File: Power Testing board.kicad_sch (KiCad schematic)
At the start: 5 parts, among them U1 INA260, U2 INA260, U3 INA260, U4 INA260

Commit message: GPT progress
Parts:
- removed A1: Arduino_Nano_Every, Module:Arduino_Nano, symbol MCU_Module:Arduino_Nano_Every
- removed U1, U2, U3, U4: INA260, Package_SO:TSSOP-16_4.4x5mm_P0.65mm, symbol Sensor:INA260
- added A1: Arduino Nano USB-powered socket, Module:Arduino_Nano, symbol Power_Testing_Board:Arduino_Nano_USB_Powered
- added C1, C3, C5, C7: 1uF input close to eFuse, Capacitor_SMD:C_0805_2012Metric, symbol Power_Testing_Board:C
- added C2, C4, C6, C8: 10uF output close to eFuse, Capacitor_SMD:C_0805_2012Metric, symbol Power_Testing_Board:C
- added J1: J_ATX_PWR: 3V3 3V3 5V 5V 12V 12V GNDx4, TerminalBlock:TerminalBlock_MaiXu_MX126-5.0-10P_1x10_P5.00mm, symbol Power_Testing_Board:Conn_01x10
- added J2: J_ATX_CTRL: PS_ON PWR_OK 5VSB GND, TerminalBlock:TerminalBlock_MaiXu_MX126-5.0-04P_1x04_P5.00mm, symbol Power_Testing_Board:Conn_01x04
- added J3: ATX_SWITCH, TerminalBlock:TerminalBlock_MaiXu_MX126-5.0-02P_1x02_P5.00mm, symbol Power_Testing_Board:Conn_01x02
- added J4: DEDICATED OUTPUTS: 3V3/G 5V/G 12V/G 16V8/G, TerminalBlock:TerminalBlock_MaiXu_MX126-5.0-08P_1x08_P5.00mm, symbol Power_Testing_Board:Conn_01x08
- added JH1: H1 selected power/GND pins only, Connector_PinSocket_2.54mm:PinSocket_2x26_P2.54mm_Vertical, symbol Power_Testing_Board:PC104_H1_SelectedPowerPins
- added JH2: H2 selected power/GND pins only, Connector_PinSocket_2.54mm:PinSocket_2x26_P2.54mm_Vertical, symbol Power_Testing_Board:PC104_H2_SelectedPowerPins
- added Q1: 2N7002 RESET_3V3 pulldown, Package_TO_SOT_SMD:SOT-23, symbol Power_Testing_Board:NMOS_GSD
- added Q2: 2N7002 RESET_5V pulldown, Package_TO_SOT_SMD:SOT-23, symbol Power_Testing_Board:NMOS_GSD
- added Q3: 2N7002 RESET_12V pulldown, Package_TO_SOT_SMD:SOT-23, symbol Power_Testing_Board:NMOS_GSD
- added Q4: 2N7002 RESET_16V8 pulldown, Package_TO_SOT_SMD:SOT-23, symbol Power_Testing_Board:NMOS_GSD
- added Q5: 2N7002 ATX PS_ON# pulldown, Package_TO_SOT_SMD:SOT-23, symbol Power_Testing_Board:NMOS_GSD
- added R1: 1.10k 1% ILM ~6A, Resistor_SMD:R_0805_2012Metric, symbol Power_Testing_Board:R
- added R10: 249k UVLO top, Resistor_SMD:R_0603_1608Metric, symbol Power_Testing_Board:R
- added R11, R19, R27: 100k UVLO bottom, Resistor_SMD:R_0603_1608Metric, symbol Power_Testing_Board:R
- added R12: 402k OVP top, Resistor_SMD:R_0603_1608Metric, symbol Power_Testing_Board:R
- added R13, R21, R29: 100k OVP bottom, Resistor_SMD:R_0603_1608Metric, symbol Power_Testing_Board:R
- added R14, R22, R30, R33, R6: 330 gate, Resistor_SMD:R_0603_1608Metric, symbol Power_Testing_Board:R
- added R15, R23, R31, R34, R7: 100k gate pulldown, Resistor_SMD:R_0603_1608Metric, symbol Power_Testing_Board:R
- added R16, R24, R32, R8: 10k FLT pullup, Resistor_SMD:R_0603_1608Metric, symbol Power_Testing_Board:R
- added R17, R25, R9: 3.00k 1% ILIM ~6A, Resistor_SMD:R_0805_2012Metric, symbol Power_Testing_Board:R
- added R18: 649k UVLO top, Resistor_SMD:R_0603_1608Metric, symbol Power_Testing_Board:R
- added R2: 100k EN top, Resistor_SMD:R_0603_1608Metric, symbol Power_Testing_Board:R
- added R20: 1.15M OVP top, Resistor_SMD:R_0603_1608Metric, symbol Power_Testing_Board:R
- added R26: 976k UVLO top, Resistor_SMD:R_0603_1608Metric, symbol Power_Testing_Board:R
- added R28: 1.50M OVP top, Resistor_SMD:R_0603_1608Metric, symbol Power_Testing_Board:R
- added R3: 100k EN bottom, Resistor_SMD:R_0603_1608Metric, symbol Power_Testing_Board:R
- added R4: 24.9k OVLO top, Resistor_SMD:R_0603_1608Metric, symbol Power_Testing_Board:R
- added R5: 10k OVLO bottom, Resistor_SMD:R_0603_1608Metric, symbol Power_Testing_Board:R
- added SW1: RESET_3V3 edge button, Button_Switch_THT:SW_PUSH_6mm, symbol Power_Testing_Board:SW_Push
- added SW2: RESET_5V edge button, Button_Switch_THT:SW_PUSH_6mm, symbol Power_Testing_Board:SW_Push
- added SW3: RESET_12V edge button, Button_Switch_THT:SW_PUSH_6mm, symbol Power_Testing_Board:SW_Push
- added SW4: RESET_16V8 edge button, Button_Switch_THT:SW_PUSH_6mm, symbol Power_Testing_Board:SW_Push
- added TP1: +3V3_RAW, TestPoint:TestPoint_Pad_D1.0mm, symbol Power_Testing_Board:TP
- added TP10: +16V8_RAW, TestPoint:TestPoint_Pad_D1.0mm, symbol Power_Testing_Board:TP
- added TP11: +16V8_EFUSE_OUT, TestPoint:TestPoint_Pad_D1.0mm, symbol Power_Testing_Board:TP
- added TP12: +16V8_PROTECTED, TestPoint:TestPoint_Pad_D1.0mm, symbol Power_Testing_Board:TP
- added TP13: GND, TestPoint:TestPoint_Pad_D1.0mm, symbol Power_Testing_Board:TP
- added TP14: I2C_SDA, TestPoint:TestPoint_Pad_D1.0mm, symbol Power_Testing_Board:TP
- added TP15: I2C_SCL, TestPoint:TestPoint_Pad_D1.0mm, symbol Power_Testing_Board:TP
- added TP16: ATX_PS_ON_N, TestPoint:TestPoint_Pad_D1.0mm, symbol Power_Testing_Board:TP
- added TP17: ATX_PWR_OK, TestPoint:TestPoint_Pad_D1.0mm, symbol Power_Testing_Board:TP
- added TP18: +5VSB, TestPoint:TestPoint_Pad_D1.0mm, symbol Power_Testing_Board:TP
- added TP19: RESET_3V3, TestPoint:TestPoint_Pad_D1.0mm, symbol Power_Testing_Board:TP
- added TP2: +3V3_EFUSE_OUT, TestPoint:TestPoint_Pad_D1.0mm, symbol Power_Testing_Board:TP
- added TP20: RESET_5V, TestPoint:TestPoint_Pad_D1.0mm, symbol Power_Testing_Board:TP
- added TP21: RESET_12V, TestPoint:TestPoint_Pad_D1.0mm, symbol Power_Testing_Board:TP
- added TP22: RESET_16V8, TestPoint:TestPoint_Pad_D1.0mm, symbol Power_Testing_Board:TP
- added TP23: FLT_3V3, TestPoint:TestPoint_Pad_D1.0mm, symbol Power_Testing_Board:TP
- added TP24: FLT_5V, TestPoint:TestPoint_Pad_D1.0mm, symbol Power_Testing_Board:TP
- added TP25: FLT_12V, TestPoint:TestPoint_Pad_D1.0mm, symbol Power_Testing_Board:TP
- added TP26: FLT_16V8, TestPoint:TestPoint_Pad_D1.0mm, symbol Power_Testing_Board:TP
- added TP27: BOOST_IN+ (+12V_RAW), TestPoint:TestPoint_Pad_D1.0mm, symbol Power_Testing_Board:TP
- added TP28: BOOST_OUT+ (+16V8_RAW), TestPoint:TestPoint_Pad_D1.0mm, symbol Power_Testing_Board:TP
- added TP29: BOOST_GND, TestPoint:TestPoint_Pad_D1.0mm, symbol Power_Testing_Board:TP
- added TP3: +3V3_PROTECTED, TestPoint:TestPoint_Pad_D1.0mm, symbol Power_Testing_Board:TP
- added TP4: +5V_RAW, TestPoint:TestPoint_Pad_D1.0mm, symbol Power_Testing_Board:TP
- added TP5: +5V_EFUSE_OUT, TestPoint:TestPoint_Pad_D1.0mm, symbol Power_Testing_Board:TP
- added TP6: +5V_PROTECTED, TestPoint:TestPoint_Pad_D1.0mm, symbol Power_Testing_Board:TP
- added TP7: +12V_RAW, TestPoint:TestPoint_Pad_D1.0mm, symbol Power_Testing_Board:TP
- added TP8: +12V_EFUSE_OUT, TestPoint:TestPoint_Pad_D1.0mm, symbol Power_Testing_Board:TP
- added TP9: +12V_PROTECTED, TestPoint:TestPoint_Pad_D1.0mm, symbol Power_Testing_Board:TP
- added U1: TPS259814L 3V3 eFuse latch-off, Package_DFN_QFN:Texas_RPU0010A_VQFN-HR-10_2x2mm_P0.5mm, symbol Power_Testing_Board:TPS259814L_RPW_eFuse
- added U2: TPS26631RGE 5V eFuse, Package_DFN_QFN:Texas_RGE0024H_VQFN-24-1EP_4x4mm_P0.5mm_EP2.7x2.7mm_ThermalVias, symbol Power_Testing_Board:TPS26631RGE_eFuse
- added U3: TPS26631RGE 12V eFuse, Package_DFN_QFN:Texas_RGE0024H_VQFN-24-1EP_4x4mm_P0.5mm_EP2.7x2.7mm_ThermalVias, symbol Power_Testing_Board:TPS26631RGE_eFuse
- added U4: TPS26631RGE 16V8 eFuse, Package_DFN_QFN:Texas_RGE0024H_VQFN-24-1EP_4x4mm_P0.5mm_EP2.7x2.7mm_ThermalVias, symbol Power_Testing_Board:TPS26631RGE_eFuse
- added U5: INA260 3V3 module, Power_Testing_Board:Adafruit_INA260_4226_Module, symbol Power_Testing_Board:Adafruit_INA260_4226_Module
- added U6: INA260 5V module, Power_Testing_Board:Adafruit_INA260_4226_Module, symbol Power_Testing_Board:Adafruit_INA260_4226_Module
- added U7: INA260 12V module, Power_Testing_Board:Adafruit_INA260_4226_Module, symbol Power_Testing_Board:Adafruit_INA260_4226_Module
- added U8: INA260 16V8 module, Power_Testing_Board:Adafruit_INA260_4226_Module, symbol Power_Testing_Board:Adafruit_INA260_4226_Module
- added U9: Boost 12V to 16.8V module 60x42 VERIFIED, Power_Testing_Board:Boost_Module_60x42_VERIFIED, symbol Power_Testing_Board:Boost_Module_60x42
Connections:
- net GND: now also A1.29 (GND), A1.4 (GND), C1.2, C2.2, C3.2, C4.2, C5.2, C6.2, C7.2, C8.2, J1.10 (Pin_10), J1.7 (Pin_7), J1.8 (Pin_8), J1.9 (Pin_9), J2.4 (Pin_4), J3.2 (Pin_2), J4.2 (Pin_2), J4.4 (Pin_4), J4.6 (Pin_6), J4.8 (Pin_8), JH1.22 (H1_22), JH1.24 (H1_24), JH1.27 (H1_27), JH1.31 (H1_31), JH1.32 (H1_32), JH1.36 (H1_36), JH1.39 (H1_39), JH1.40 (H1_40), JH1.42 (H1_42), JH2.29 (H2_29), JH2.30 (H2_30), JH2.31 (H2_31), JH2.32 (H2_32), JH2.36 (H2_36), JH2.39 (H2_39), JH2.40 (H2_40), JH2.41 (H2_41), JH2.42 (H2_42), JH2.43 (H2_43), JH2.44 (H2_44), Q1.2 (S), Q2.2 (S), Q3.2 (S), Q4.2 (S), Q5.2 (S), R1.2, R11.2, R13.2, R15.2, R17.2, R19.2, R21.2, R23.2, R25.2, R27.2, R29.2, R3.2, R31.2, R34.2, R5.2, R7.2, R9.2, SW1.2, SW2.2, SW3.2, SW4.2, TP13.1 (TP), TP29.1 (TP), U1.8 (GND), U2.25 (EP_GND), U2.8 (GND), U3.25 (EP_GND), U3.8 (GND), U4.25 (EP_GND), U4.8 (GND), U5.2 (GND), U6.2 (GND), U7.2 (GND), U8.2 (GND), U9.1 (IN-), U9.3 (OUT-)
- new net +12V_EFUSE_OUT: C6.1, TP8.1 (TP), U3.17 (OUT), U3.18 (OUT), U7.7 (VIN+)
- new net +12V_PROTECTED: J4.5 (Pin_5), JH1.52 (H1_52), TP9.1 (TP), U7.8 (VIN-)
- new net +12V_RAW: C5.1, J1.5 (Pin_5), J1.6 (Pin_6), R18.1, R20.1, TP27.1 (TP), TP7.1 (TP), U3.1 (IN), U3.2 (IN), U3.5 (IN_SYS), U9.2 (IN+)
- new net +16V8_EFUSE_OUT: C8.1, TP11.1 (TP), U4.17 (OUT), U4.18 (OUT), U8.7 (VIN+)
- new net +16V8_PROTECTED: J4.7 (Pin_7), JH2.45 (H2_45), JH2.46 (H2_46), TP12.1 (TP), U8.8 (VIN-)
- new net +16V8_RAW: C7.1, R26.1, R28.1, TP10.1 (TP), TP28.1 (TP), U4.1 (IN), U4.2 (IN), U4.5 (IN_SYS), U9.4 (OUT+)
- new net +3V3_EFUSE_OUT: C2.1, TP2.1 (TP), U1.6 (OUT), U5.7 (VIN+)
- new net +3V3_PROTECTED: J4.1 (Pin_1), JH1.48 (H1_48), JH2.27 (H2_27), JH2.28 (H2_28), TP3.1 (TP), U5.8 (VIN-)
- new net +3V3_RAW: C1.1, J1.1 (Pin_1), J1.2 (Pin_2), R2.1, R4.1, TP1.1 (TP), U1.5 (IN)
- new net +5VSB: J2.3 (Pin_3), TP18.1 (TP)
- new net +5V_EFUSE_OUT: C4.1, TP5.1 (TP), U2.17 (OUT), U2.18 (OUT), U6.7 (VIN+)
- new net +5V_PROTECTED: J4.3 (Pin_3), JH1.47 (H1_47), JH1.49 (H1_49), JH2.25 (H2_25), JH2.26 (H2_26), TP6.1 (TP), U6.8 (VIN-)
- new net +5V_RAW: C3.1, J1.3 (Pin_3), J1.4 (Pin_4), R10.1, R12.1, TP4.1 (TP), U2.1 (IN), U2.2 (IN), U2.5 (IN_SYS)
- new net +ARDUINO_5V: A1.27 (5V), R16.2, R24.2, R32.2, R8.2, U5.1 (VCC), U6.1 (VCC), U7.1 (VCC), U8.1 (VCC)
- new net ALERT_12V: U7.5 (ALERT)
- new net ALERT_16V8: U8.5 (ALERT)
- new net ALERT_3V3: U5.5 (ALERT)
- new net ALERT_5V: U6.5 (ALERT)
- new net ARD_RESET_12V: A1.7 (D4), R22.1
- new net ARD_RESET_16V8: A1.8 (D5), R30.1
- new net ARD_RESET_3V3: A1.5 (D2), R6.1
- new net ARD_RESET_5V: A1.6 (D3), R14.1
- new net ATX_PS_ON_CTL: A1.13 (D10), R33.1
- new net ATX_PS_ON_N: J2.1 (Pin_1), J3.1 (Pin_1), Q5.3 (D), TP16.1 (TP)
- new net ATX_PWR_OK: A1.14 (D11), J2.2 (Pin_2), TP17.1 (TP)
- new net FLT_12V: A1.11 (D8), R24.1, TP25.1 (TP), U3.14 (~FLT)
- new net FLT_16V8: A1.12 (D9), R32.1, TP26.1 (TP), U4.14 (~FLT)
- new net FLT_3V3: A1.9 (D6), R8.1, TP23.1 (TP), U1.4 (~FLT)
- new net FLT_5V: A1.10 (D7), R16.1, TP24.1 (TP), U2.14 (~FLT)
- new net GATE_12V: Q3.1 (G), R22.2, R23.1
- new net GATE_16V8: Q4.1 (G), R30.2, R31.1
- new net GATE_3V3: Q1.1 (G), R6.2, R7.1
- new net GATE_5V: Q2.1 (G), R14.2, R15.1
- new net GATE_PS_ON: Q5.1 (G), R33.2, R34.1
- new net I2C_SCL: A1.24 (A5/SCL), TP15.1 (TP), U5.3 (SCL), U6.3 (SCL), U7.3 (SCL), U8.3 (SCL)
- new net I2C_SDA: A1.23 (A4/SDA), TP14.1 (TP), U5.4 (SDA), U6.4 (SDA), U7.4 (SDA), U8.4 (SDA)
- new net ILIM_12V: R17.1, U3.10 (ILIM)
- new net ILIM_16V8: R25.1, U4.10 (ILIM)
- new net ILIM_3V3: R1.1, U1.9 (ILM)
- new net ILIM_5V: R9.1, U2.10 (ILIM)
- new net IMON_12V: U3.13 (IMON)
- new net IMON_16V8: U4.13 (IMON)
- new net IMON_5V: U2.13 (IMON)
- new net OVLO_3V3: R4.2, R5.1, U1.2 (EN/OVLO)
- new net OVP_12V: R20.2, R21.1, U3.7 (OVP)
- new net OVP_16V8: R28.2, R29.1, U4.7 (OVP)
- new net OVP_5V: R12.2, R13.1, U2.7 (OVP)
- new net PG_12V: U3.16 (PGOOD)
- new net PG_16V8: U4.16 (PGOOD)
- new net PG_3V3: U1.3 (PG)
- new net PG_5V: U2.16 (PGOOD)
- new net RESET_12V: Q3.3 (D), SW3.1, TP21.1 (TP), U3.12 (~SHDN)
- new net RESET_16V8: Q4.3 (D), SW4.1, TP22.1 (TP), U4.12 (~SHDN)
- new net RESET_3V3: Q1.3 (D), R2.2, R3.1, SW1.1, TP19.1 (TP), U1.1 (EN/UVLO)
- new net RESET_5V: Q2.3 (D), SW2.1, TP20.1 (TP), U2.12 (~SHDN)
- new net UVLO_12V: R18.2, R19.1, U3.6 (UVLO)
- new net UVLO_16V8: R26.2, R27.1, U4.6 (UVLO)
- new net UVLO_5V: R10.2, R11.1, U2.6 (UVLO)
- no-connect marks 0 -> 25
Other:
- removed sheet Headers
- removed sheet Untitled Sheet
- note added: "Boost module footprint uses physically verified 60 mm x 42 mm x 20 mm module geometry."
- note added: "Compact layout choice: eFuse ICs are on the main PCB for minimum size. If field replacement becomes more important than area, move each eFuse circuit to a plug-in daughterboard."
- note added: "Only user-selected H1/H2 mission power and GND pins are connected. Excluded/communication pins are not represented in this schematic."
- note added: "Power path on every rail: RAW -> eFuse -> INA260 VIN+ -> INA260 VIN- -> PROTECTED output. INA260 VIN- is the downstream positive rail, never GND."
- title: Power Testing Board -> Compact CubeSat EPS Power Testing Board

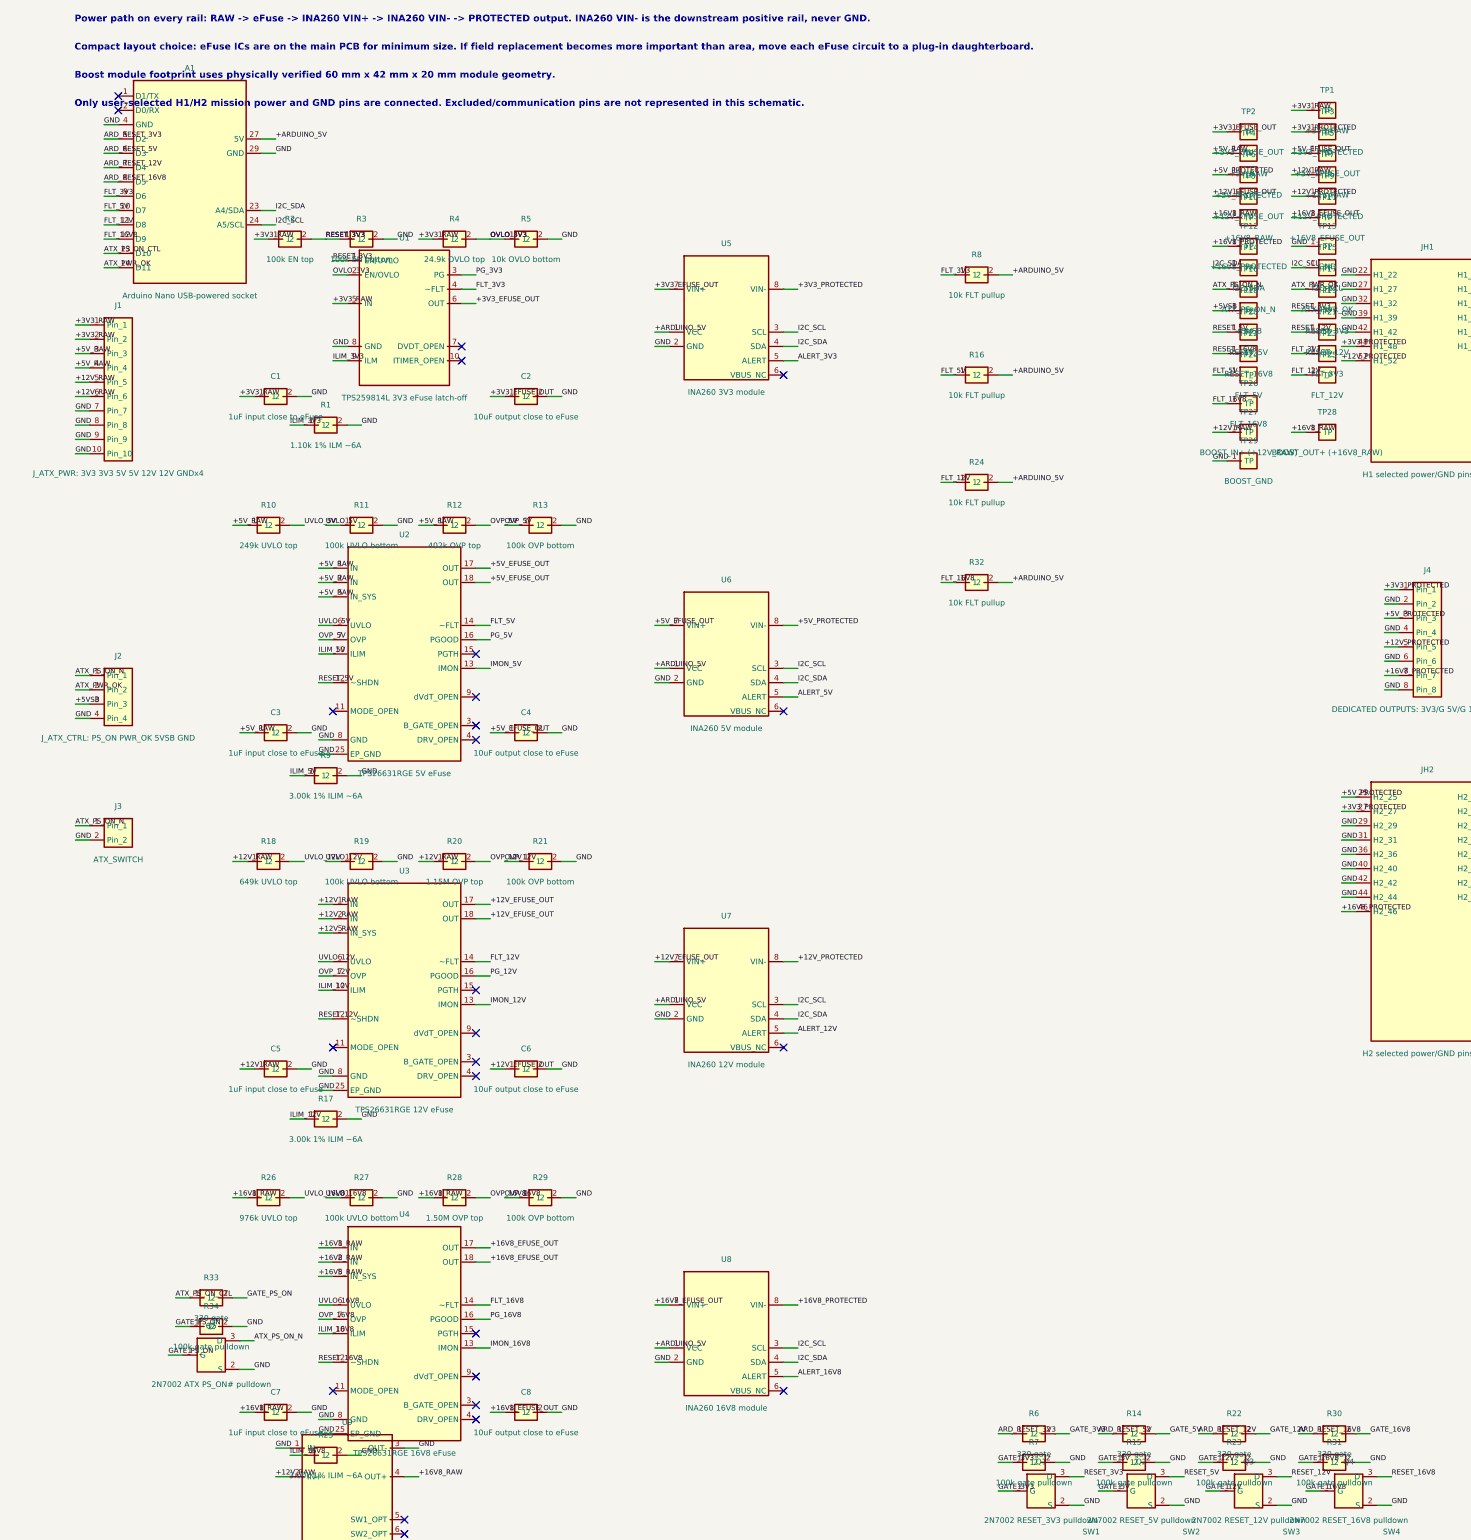
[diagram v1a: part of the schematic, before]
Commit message: chat gpt pt.2
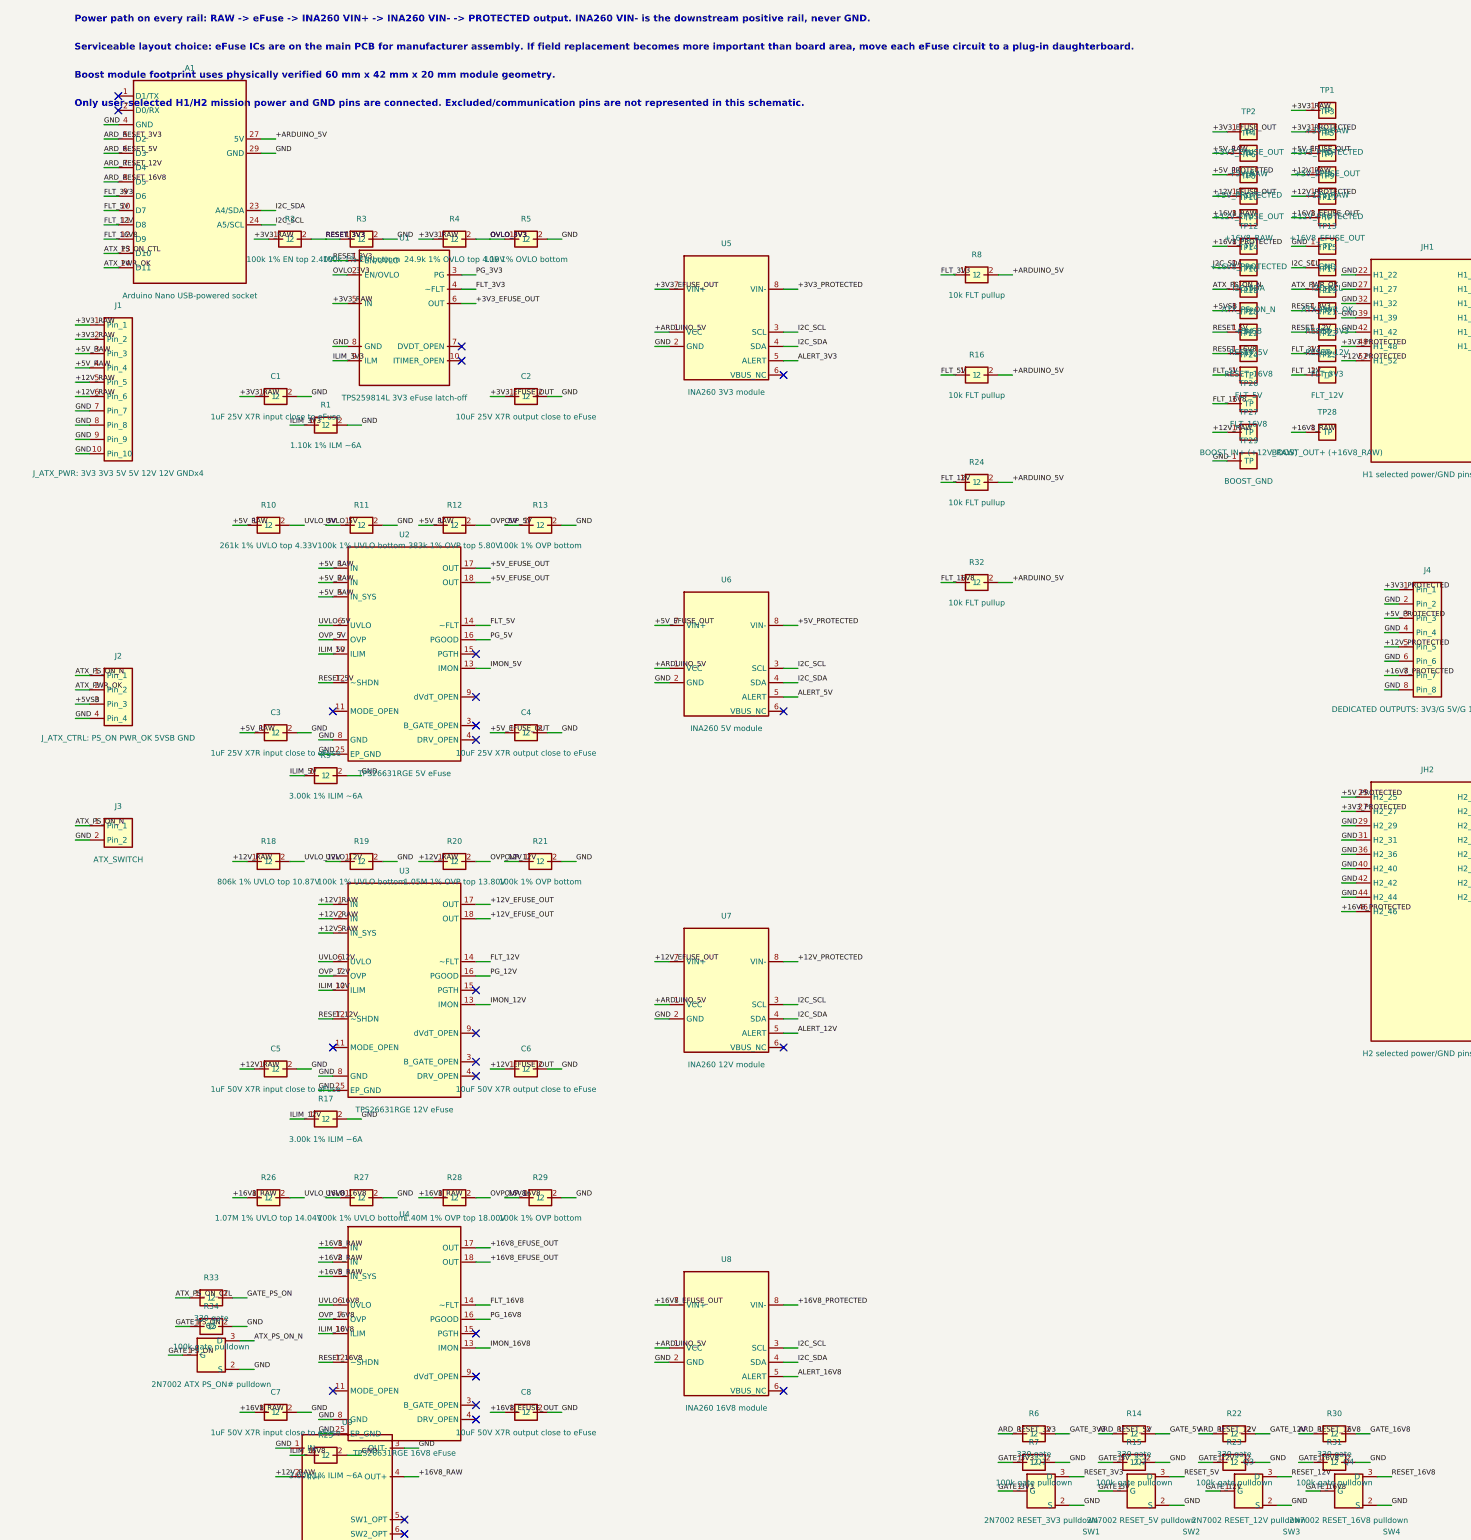
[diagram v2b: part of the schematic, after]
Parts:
- C1, C3: value 1uF input close to eFuse -> 1uF 25V X7R input close to eFuse
- C2, C4: value 10uF output close to eFuse -> 10uF 25V X7R output close to eFuse
- C5, C7: value 1uF input close to eFuse -> 1uF 50V X7R input close to eFuse
- C6, C8: value 10uF output close to eFuse -> 10uF 50V X7R output close to eFuse
- R10: value 249k UVLO top -> 261k 1% UVLO top 4.33V
- R11, R19, R27: value 100k UVLO bottom -> 100k 1% UVLO bottom
- R12: value 402k OVP top -> 383k 1% OVP top 5.80V
- R13, R21, R29: value 100k OVP bottom -> 100k 1% OVP bottom
- R18: value 649k UVLO top -> 806k 1% UVLO top 10.87V
- R2: value 100k EN top -> 100k 1% EN top 2.40V
- R20: value 1.15M OVP top -> 1.05M 1% OVP top 13.80V
- R26: value 976k UVLO top -> 1.07M 1% UVLO top 14.04V
- R28: value 1.50M OVP top -> 1.40M 1% OVP top 18.00V
- R3: value 100k EN bottom -> 100k 1% EN bottom
- R4: value 24.9k OVLO top -> 24.9k 1% OVLO top 4.19V
- R5: value 10k OVLO bottom -> 10k 1% OVLO bottom
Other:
- note added: "Serviceable layout choice: eFuse ICs are on the main PCB for manufacturer assembly. If field replacement becomes more important than board area, move each eFuse circuit to a plug-in daughterboard."
- note removed: "Compact layout choice: eFuse ICs are on the main PCB for minimum size. If field replacement becomes more important than area, move each eFuse circuit to a plug-in daughterboard."
